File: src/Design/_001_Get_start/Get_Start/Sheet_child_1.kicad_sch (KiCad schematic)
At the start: 0 parts

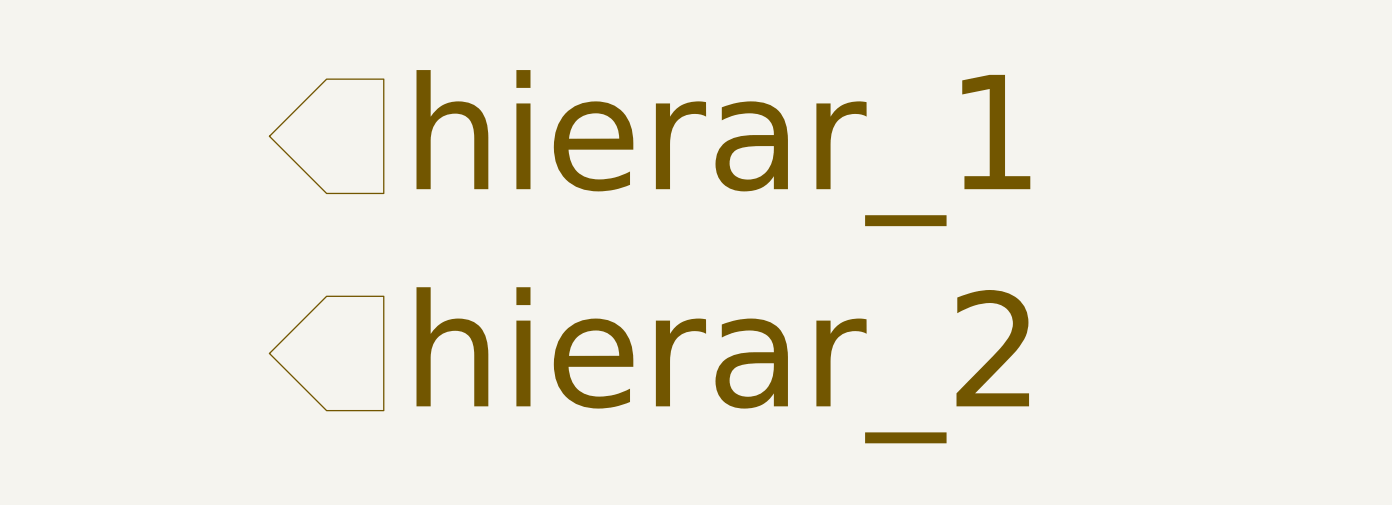
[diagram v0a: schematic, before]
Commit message: reup
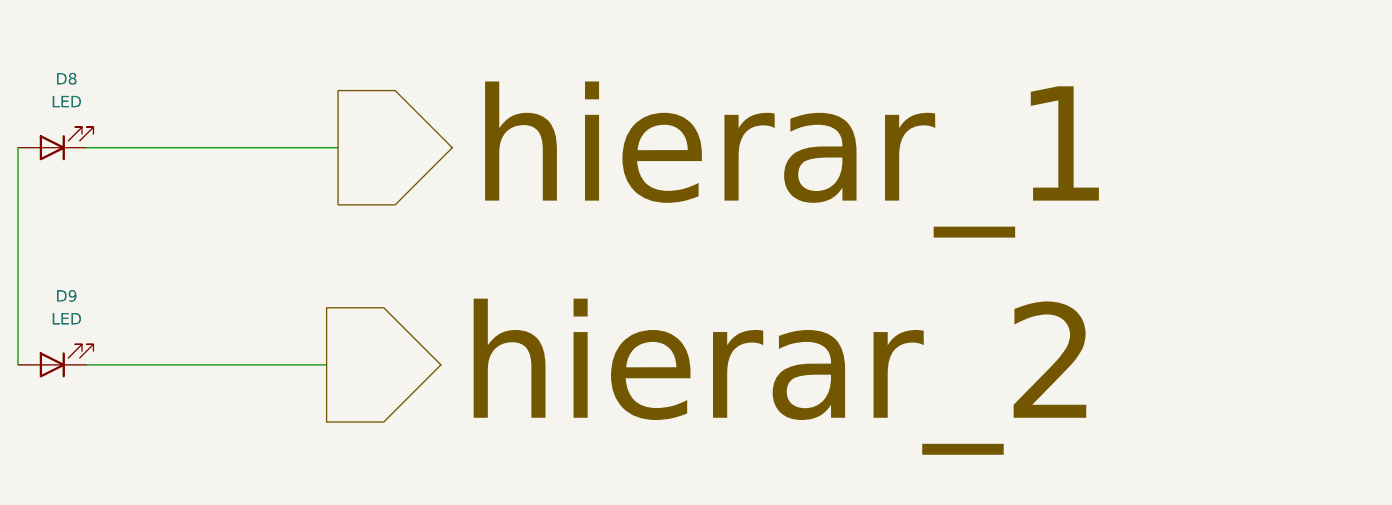
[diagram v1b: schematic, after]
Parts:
- added D8, D9: LED, symbol Device:LED
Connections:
- net hierar_1: now also D8.1 (K)
- net hierar_2: now also D9.1 (K)
- new net: D8.2 (A), D9.2 (A)
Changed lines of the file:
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@@
 	(generator_version "9.0")
 	(paper "A4")
+	(wire
+		(pts
+			(xy 50.8 44.45) (xy 78.74 44.45)
+		)
+		(stroke
+			(width 0)
+			(type default)
+		)
+	)
+	(wire
+		(pts
+			(xy 43.18 44.45) (xy 43.18 68.58)
+		)
+		(stroke
+			(width 0)
+			(type default)
+		)
+	)
+	(wire
+		(pts
+			(xy 50.8 68.58) (xy 77.47 68.58)
+		)
+		(stroke
+			(width 0)
+			(type default)
+		)
+	)
 	(hierarchical_label "hierar_2"
-		(shape input)
-		(at 71.12 67.31 0)
+		(shape output)
+		(at 77.47 68.58 0)
 		(effects
 			(font
@@
 	)
 	(hierarchical_label "hierar_1"
-		(shape input)
-		(at 71.12 43.18 0)
+		(shape output)
+		(at 78.74 44.45 0)
 		(effects
 			(font
@@
 		)
 	)
+	(symbol
+		(lib_id "Device:LED")
+		(at 46.99 44.45 180)
+		(unit 1)
+		(exclude_from_sim no)
+		(in_bom yes)
+		(on_board yes)
+		(dnp no)
+		(fields_autoplaced yes)
+		(property "Reference" "D8"
+			(at 48.5775 36.83 0)
+			(effects
+				(font
+					(size 1.27 1.27)
+				)
+			)
+		)
+		(property "Value" "LED"
+			(at 48.5775 39.37 0)
+			(effects
+				(font
+					(size 1.27 1.27)
+				)
+			)
+		)
+		(property "Footprint" ""
+			(at 46.99 44.45 0)
+			(effects
+				(font
+					(size 1.27 1.27)
+				)
+				(hide yes)
+			)
+		)
+		(property "Datasheet" "~"
+			(at 46.99 44.45 0)
+			(effects
+				(font
+					(size 1.27 1.27)
+				)
+				(hide yes)
+			)
+		)
+		(property "Description" "Light emitting diode"
+			(at 46.99 44.45 0)
+			(effects
+				(font
+					(size 1.27 1.27)
+				)
+				(hide yes)
+			)
+		)
+		(property "Sim.Pins" "1=K 2=A"
+			(at 46.99 44.45 0)
+			(effects
+				(font
+					(size 1.27 1.27)
+				)
+				(hide yes)
+			)
+		)
+		(pin "2"
+		)
+		(pin "1"
+		)
+		(instances
+			(project ""
+				(path "/3c26b505-18dc-433f-8569-20dcedbd6448/40e9da73-9318-4acd-848a-baa96530663d"
+					(reference "D8")
+					(unit 1)
+				)
+			)
+		)
+	)
+	(symbol
+		(lib_id "Device:LED")
+		(at 46.99 68.58 180)
+		(unit 1)
+		(exclude_from_sim no)
+		(in_bom yes)
+		(on_board yes)
+		(dnp no)
+		(fields_autoplaced yes)
+		(property "Reference" "D9"
+			(at 48.5775 60.96 0)
+			(effects
+				(font
+					(size 1.27 1.27)
+				)
+			)
+		)
+		(property "Value" "LED"
+			(at 48.5775 63.5 0)
+			(effects
+				(font
+					(size 1.27 1.27)
+				)
+			)
+		)
+		(property "Footprint" ""
+			(at 46.99 68.58 0)
+			(effects
+				(font
+					(size 1.27 1.27)
+				)
+				(hide yes)
+			)
+		)
+		(property "Datasheet" "~"
+			(at 46.99 68.58 0)
+			(effects
+				(font
+					(size 1.27 1.27)
+				)
+				(hide yes)
+			)
+		)
+		(property "Description" "Light emitting diode"
+			(at 46.99 68.58 0)
+			(effects
+				(font
+					(size 1.27 1.27)
+				)
+				(hide yes)
+			)
+		)
+		(property "Sim.Pins" "1=K 2=A"
+			(at 46.99 68.58 0)
+			(effects
+				(font
+					(size 1.27 1.27)
+				)
+				(hide yes)
+			)
+		)
+		(pin "2"
+		)
+		(pin "1"
+		)
+		(instances
+			(project ""
+				(path "/3c26b505-18dc-433f-8569-20dcedbd6448/40e9da73-9318-4acd-848a-baa96530663d"
+					(reference "D9")
+					(unit 1)
+				)
+			)
+		)
+	)
